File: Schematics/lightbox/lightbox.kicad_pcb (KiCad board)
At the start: 2 copper layers, 5 parts, among them J3 Conn_01x12_Female, U5 D148K, U6 D148K, U7 D148K, U8 D148K

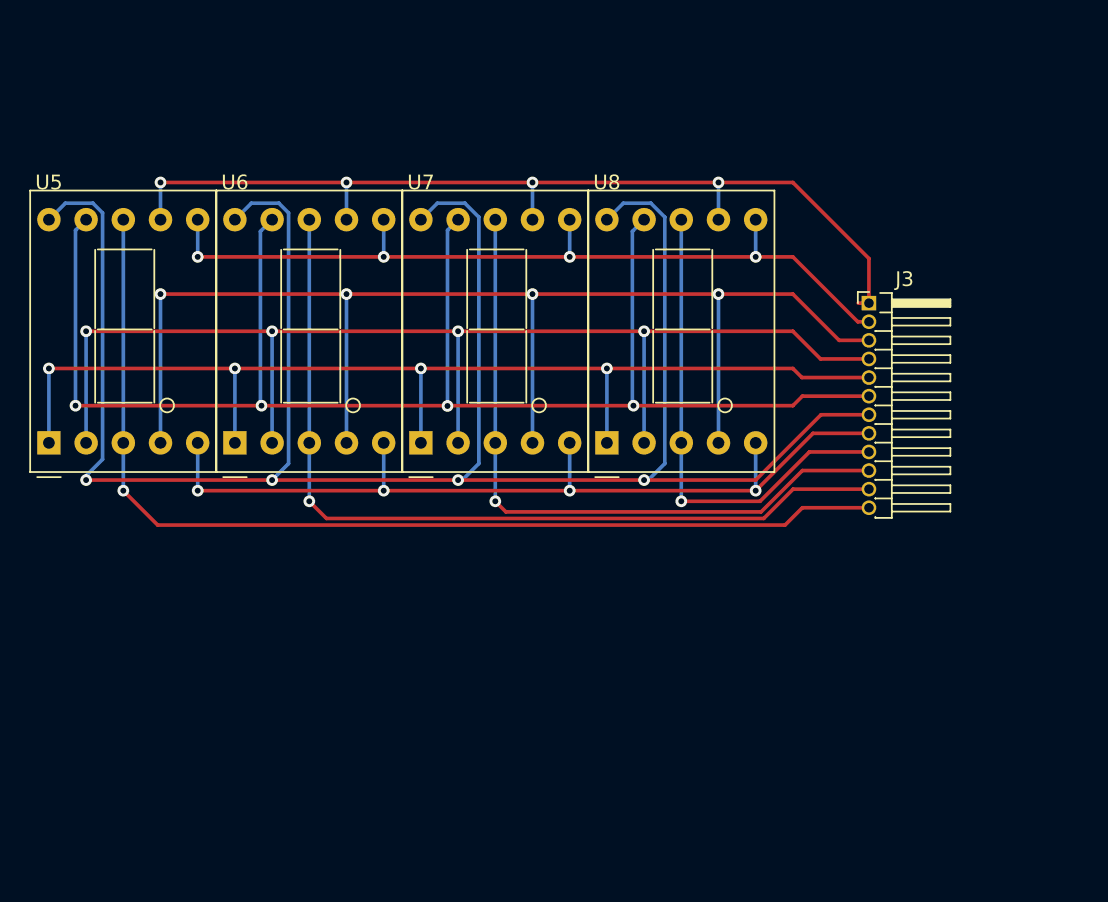
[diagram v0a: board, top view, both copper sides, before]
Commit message: Update Schematic and PCB layout
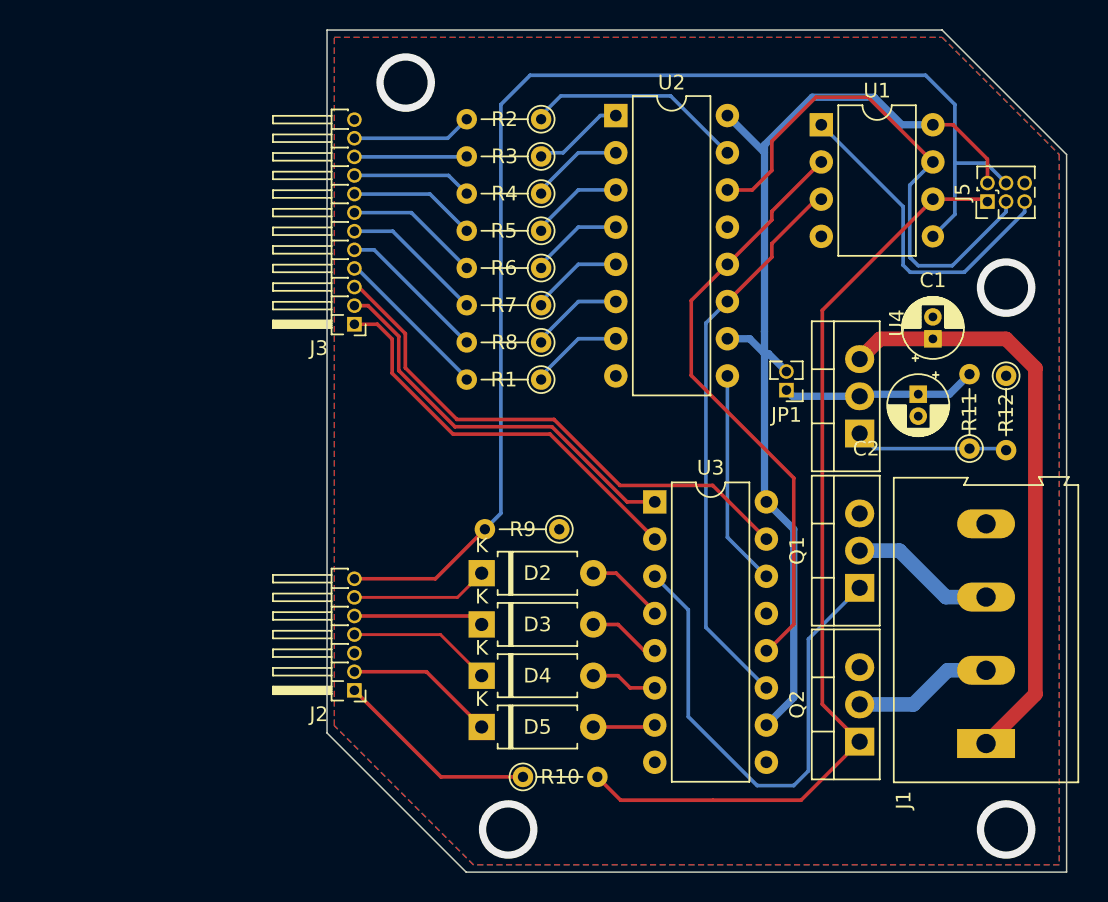
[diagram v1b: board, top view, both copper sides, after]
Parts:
- removed U5, U6, U7, U8: D148K, Display_7Segment:D1X8K
- added C1: 0.1µF, Capacitor_THT:CP_Radial_D4.0mm_P1.50mm, F.Cu at (164.5, 94.5)
- added C2: 10µF, Capacitor_THT:CP_Radial_D4.0mm_P1.50mm, F.Cu at (163.5, 98.3)
- added D2: D, Diode_THT:D_A-405_P7.62mm_Horizontal, F.Cu at (133.7, 110.5)
- added D3: D, Diode_THT:D_A-405_P7.62mm_Horizontal, F.Cu at (133.7, 114.0)
- added D4: D, Diode_THT:D_A-405_P7.62mm_Horizontal, F.Cu at (133.7, 117.5)
- added D5: D, Diode_THT:D_A-405_P7.62mm_Horizontal, F.Cu at (133.7, 121.0)
- added J1: Screw_Terminal_01x04, TerminalBlock:TerminalBlock_Altech_AK300-4_P5.00mm, F.Cu at (168.1, 122.1)
- added J2: Conn_01x07_Female, Connector_PinHeader_1.27mm:PinHeader_1x07_P1.27mm_Horizontal, F.Cu at (125.0, 118.5)
- added J5: Conn_02x03_Odd_Even, Connector_PinHeader_1.27mm:PinHeader_2x03_P1.27mm_Vertical, F.Cu at (168.2, 85.1)
- added JP1: Jumper_2_Bridged, Connector_PinHeader_1.27mm:PinHeader_1x02_P1.27mm_Vertical, F.Cu at (154.5, 98.0)
- added Q1: IRF740, Package_TO_SOT_THT:TO-220-3_Vertical, F.Cu at (159.5, 111.5)
- added Q2: IRF740, Package_TO_SOT_THT:TO-220-3_Vertical, F.Cu at (159.5, 122.0)
- added R1: 470R, Resistor_THT:R_Axial_DIN0204_L3.6mm_D1.6mm_P5.08mm_Vertical, F.Cu at (137.8, 97.3)
- added R10: 470R, Resistor_THT:R_Axial_DIN0204_L3.6mm_D1.6mm_P5.08mm_Vertical, F.Cu at (136.5, 124.4)
- added R11: 1K, Resistor_THT:R_Axial_DIN0204_L3.6mm_D1.6mm_P5.08mm_Vertical, F.Cu at (167.0, 102.0)
- added R12: 1.5K, Resistor_THT:R_Axial_DIN0204_L3.6mm_D1.6mm_P5.08mm_Vertical, F.Cu at (169.5, 97.0)
- added R2: 470R, Resistor_THT:R_Axial_DIN0204_L3.6mm_D1.6mm_P5.08mm_Vertical, F.Cu at (137.8, 79.5)
- added R3: 470R, Resistor_THT:R_Axial_DIN0204_L3.6mm_D1.6mm_P5.08mm_Vertical, F.Cu at (137.8, 82.0)
- added R4: 470R, Resistor_THT:R_Axial_DIN0204_L3.6mm_D1.6mm_P5.08mm_Vertical, F.Cu at (137.8, 84.6)
- added R5: 470R, Resistor_THT:R_Axial_DIN0204_L3.6mm_D1.6mm_P5.08mm_Vertical, F.Cu at (137.8, 87.1)
- added R6: 470R, Resistor_THT:R_Axial_DIN0204_L3.6mm_D1.6mm_P5.08mm_Vertical, F.Cu at (137.8, 89.7)
- added R7: 470R, Resistor_THT:R_Axial_DIN0204_L3.6mm_D1.6mm_P5.08mm_Vertical, F.Cu at (137.8, 92.2)
- added R8: 470R, Resistor_THT:R_Axial_DIN0204_L3.6mm_D1.6mm_P5.08mm_Vertical, F.Cu at (137.8, 94.7)
- added R9: 1K, Resistor_THT:R_Axial_DIN0204_L3.6mm_D1.6mm_P5.08mm_Vertical, F.Cu at (139.0, 107.5)
- added U1: ATtiny85-20P, Package_DIP:DIP-8_W7.62mm, F.Cu at (156.9, 79.9)
- added U2: 74AHCT595, Package_DIP:DIP-16_W7.62mm, F.Cu at (142.8, 79.2)
- added U3: 74HC595, Package_DIP:DIP-16_W7.62mm, F.Cu at (145.5, 105.6)
- added U4: LM317_TO-220, Package_TO_SOT_THT:TO-220-3_Vertical, F.Cu at (159.5, 101.0)
- J3: value Conn_01x12_Female -> Conn_01x11_Female
- moved J3 35.2 mm to (125.0, 93.5), turned to 180 degrees
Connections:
- J3 pad 1: /A -> /Digit3
- J3 pad 10: /Digit3 -> /B
- J3 pad 11: /Digit2 -> /A
- J3 pad 12: /Digit1 -> (no net)
- J3 pad 2: /B -> /Digit2
- J3 pad 3: /C -> /Digit1
- J3 pad 4: /D -> /H
- J3 pad 5: /E -> /G
- J3 pad 7: /G -> /E
- J3 pad 8: /H -> /D
- J3 pad 9: /Digit4 -> /C
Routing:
- net /G: track 148.6 -> 10.3 mm, vias 4 -> 0
- net /F: track 106.6 -> 9.76 mm, vias 4 -> 0
- net /Keypad: track 0.00 -> 86.1 mm
- net /C: track 90.3 -> 8.18 mm, vias 4 -> 0
- net /D: track 84.7 -> 8.71 mm, vias 4 -> 0
- net +3V3: track 0.00 -> 69.7 mm
- net /E: track 76.6 -> 9.24 mm, vias 4 -> 0
- net /UVLeds: track 0.00 -> 65.2 mm
- net /A: track 64.5 -> 8.21 mm, vias 4 -> 0
- net /B: track 57.8 -> 7.68 mm, vias 4 -> 0
- net /H: track 60.5 -> 10.9 mm, vias 4 -> 0
- net /Rclk: track 0.00 -> 40.8 mm
- net +12V: track 0.00 -> 40.4 mm
- net /Clk: track 0.00 -> 38.5 mm
- net /Data: track 0.00 -> 35.8 mm
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- added copper zone on B.Cu, net GND
- added copper zone on F.Cu, net GND
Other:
- board outline added: 50.5 x 57.5 mm
